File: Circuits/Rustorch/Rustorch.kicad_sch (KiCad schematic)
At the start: 57 parts, among them CN1 USB_C_Receptacle_USB2.0_16P, CN2 OLED_128x64_IIC, Q1 2SC1815, Q2 2SC1815, Q3 2SC1815, Q4 2SC1815, SW1 ToggleSW 3P, SW2 RESET, SW3 SW_BOOT, SW4 SW_UP, SW5 SW_LEFT, SW6 SW_RIGHT, SW7 SW_DOWN, SW8 SW_A, SW9 SW_B, U1 ESP32-C6-WROOM-1, U2 BA033CC0T, U3 OSL10561-L*, U4 OSL10561-L*, U5 OSL10561-L*, U6 OSL10561-L*

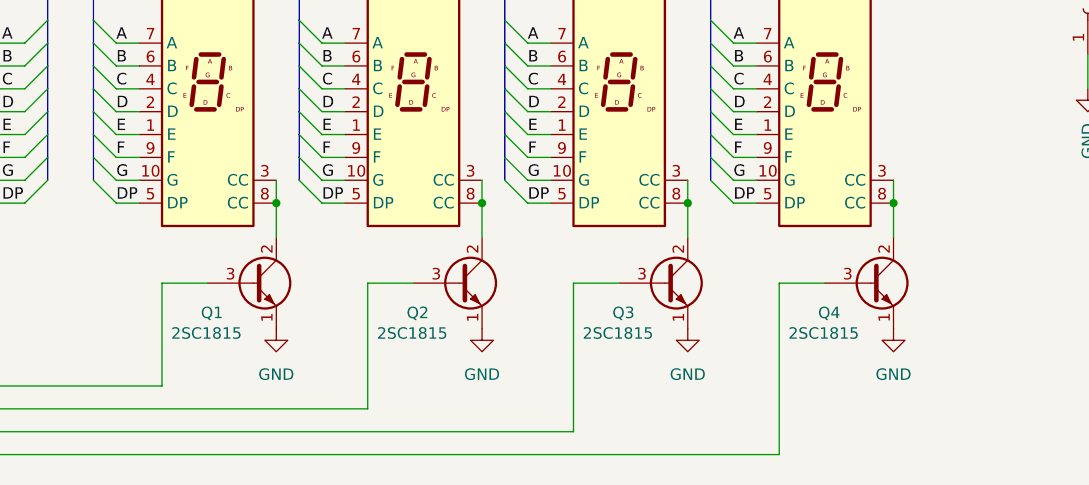
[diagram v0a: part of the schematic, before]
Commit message: (Rustorch) 配線作業 (4層化)
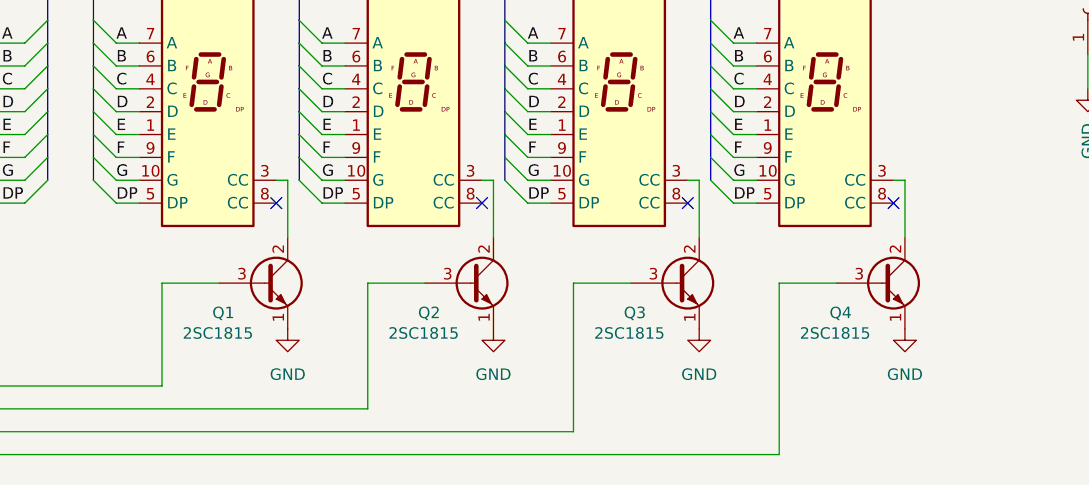
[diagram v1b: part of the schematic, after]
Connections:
- net at Q4.2 (C), U6.3 (CC): no longer U6.8 (CC)
- net at Q3.2 (C), U5.3 (CC): no longer U5.8 (CC)
- net at Q1.2 (C), U3.3 (CC): no longer U3.8 (CC)
- net at Q2.2 (C), U4.3 (CC): no longer U4.8 (CC)
- no-connect marks 5 -> 9
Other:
- moved on the sheet: Q1, Q2, Q3, Q4
